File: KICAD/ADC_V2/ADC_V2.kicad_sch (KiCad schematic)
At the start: 35 parts, among them J1 Conn_01x08_Pin, J2 Conn_01x01_Pin, J3 Conn_01x03, J5 Conn_01x01_Pin, J6 Conn_01x04, J7 Conn_01x04, J9 Conn_01x02_Pin, U3 TLV320ADC6140, U4 MIC5219-3.3YM5

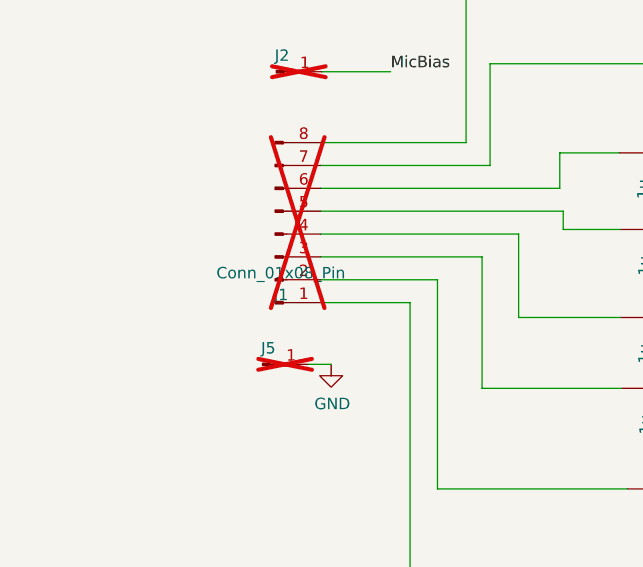
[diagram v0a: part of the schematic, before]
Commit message: v19-12-24
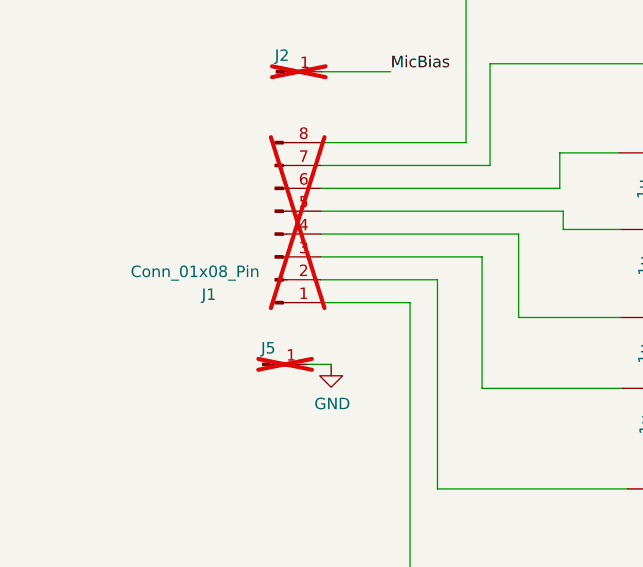
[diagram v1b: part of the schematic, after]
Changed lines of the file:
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@@
 		(dnp yes)
 		(property "Reference" "J1"
-			(at 60.325 80.5475 0)
+			(at 52.324 80.518 0)
 			(effects
 				(font
@@
 		)
 		(property "Value" "Conn_01x08_Pin"
-			(at 60.325 78.1233 0)
+			(at 50.8 77.978 0)
 			(effects
 				(font

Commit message: v07-10-25
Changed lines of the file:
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@@
 (kicad_sch
-	(version 20231120)
+	(version 20250114)
 	(generator "eeschema")
-	(generator_version "8.0")
+	(generator_version "9.0")
 	(paper "A4")
 	(title_block
@@
 		(company "WMXZ")
 	)
+	(text "https://www.allaboutcircuits.com/technical-articles/clean-power-for-every-ic-part-1-understanding-bypass-capacitors/"
+		(exclude_from_sim no)
+		(at 31.115 166.497 0)
+		(effects
+			(font
+				(size 1.27 1.27)
+			)
+			(justify left bottom)
+		)
+	)
 	(junction
 		(at 163.322 50.673)
@@
 		)
 	)
-	(text "https://www.allaboutcircuits.com/technical-articles/clean-power-for-every-ic-part-1-understanding-bypass-capacitors/"
-		(exclude_from_sim no)
-		(at 31.115 166.497 0)
-		(effects
-			(font
-				(size 1.27 1.27)
-			)
-			(justify left bottom)
-		)
-	)
 	(label "VIN"
 		(at 99.441 130.048 0)
-		(fields_autoplaced yes)
 		(effects
 			(font
@@
 	(label "VIN_EN"
 		(at 224.282 127.508 0)
-		(fields_autoplaced yes)
 		(effects
 			(font
@@
 	(label "GPIO1"
 		(at 176.53 115.57 0)
-		(fields_autoplaced yes)
 		(effects
 			(font
@@
 	(label "SCL"
 		(at 178.435 82.55 0)
-		(fields_autoplaced yes)
 		(effects
 			(font
@@
 	(label "MicBias"
 		(at 72.517 55.753 0)
-		(fields_autoplaced yes)
 		(effects
 			(font
@@
 	(label "AVDD"
 		(at 195.961 128.651 0)
-		(fields_autoplaced yes)
 		(effects
 			(font
@@
 	(label "GND"
 		(at 195.961 126.111 0)
-		(fields_autoplaced yes)
 		(effects
 			(font
@@
 	(label "SHDNZ"
 		(at 178.435 87.63 0)
-		(fields_autoplaced yes)
 		(effects
 			(font
@@
 	(label "MicBias"
 		(at 133.35 58.42 0)
-		(fields_autoplaced yes)
 		(effects
 			(font
@@
 	(label "AVDD"
 		(at 165.354 127.508 0)
-		(fields_autoplaced yes)
 		(effects
 			(font
@@
 	(label "BCLK"
 		(at 178.435 72.39 0)
-		(fields_autoplaced yes)
 		(effects
 			(font
@@
 	(label "AVDD"
 		(at 208.153 50.673 0)
-		(fields_autoplaced yes)
 		(effects
 			(font
@@
 	(label "FSYNC"
 		(at 178.435 69.85 0)
-		(fields_autoplaced yes)
 		(effects
 			(font
@@
 	(label "VIN_EN"
 		(at 122.047 132.588 0)
-		(fields_autoplaced yes)
 		(effects
 			(font
@@
 	(label "SDOUT"
 		(at 178.435 74.93 0)
-		(fields_autoplaced yes)
 		(effects
 			(font
@@
 	(label "VIN"
 		(at 217.551 130.048 0)
-		(fields_autoplaced yes)
 		(effects
 			(font
@@
 	(label "IOVD"
 		(at 208.28 61.595 0)
-		(fields_autoplaced yes)
 		(effects
 			(font
@@
 	(label "SDA"
 		(at 178.435 80.01 0)
-		(fields_autoplaced yes)
 		(effects
 			(font
@@
 		)
 	)
+	(embedded_fonts no)
 )
